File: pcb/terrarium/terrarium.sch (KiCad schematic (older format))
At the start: 22 parts, among them J3 Screw_Terminal_01x03, K3 SANYOU_SRD_Form_C, Q2 MMBT3904, U2 MOC3020M

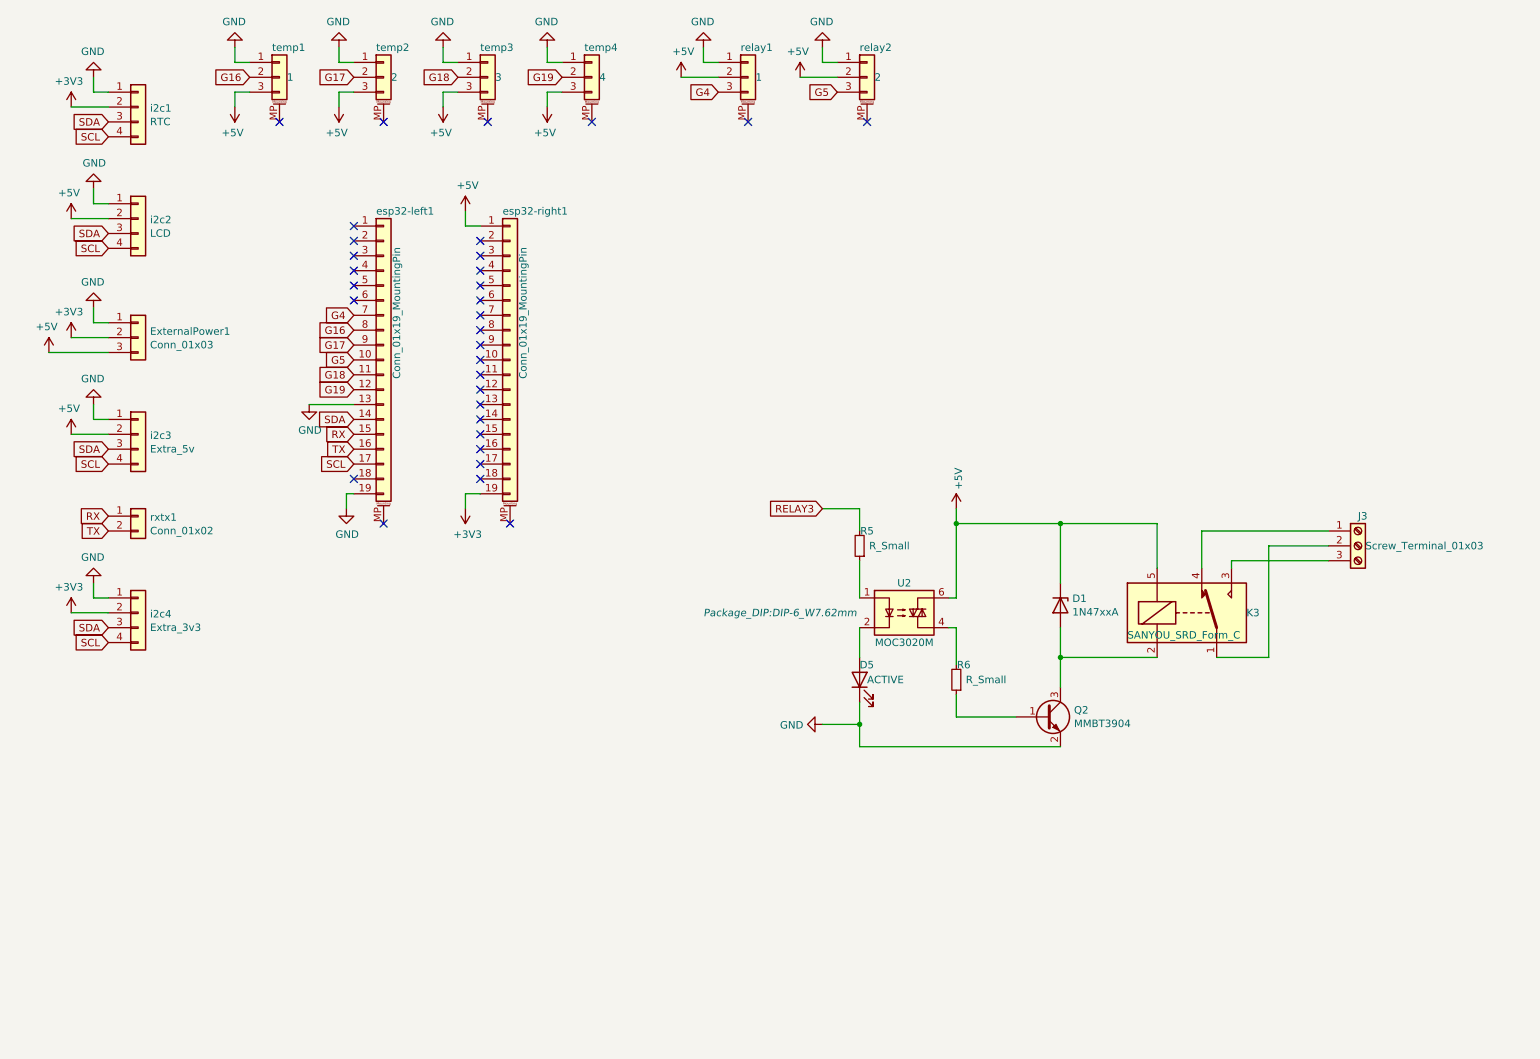
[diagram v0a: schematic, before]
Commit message: wip: update pcb
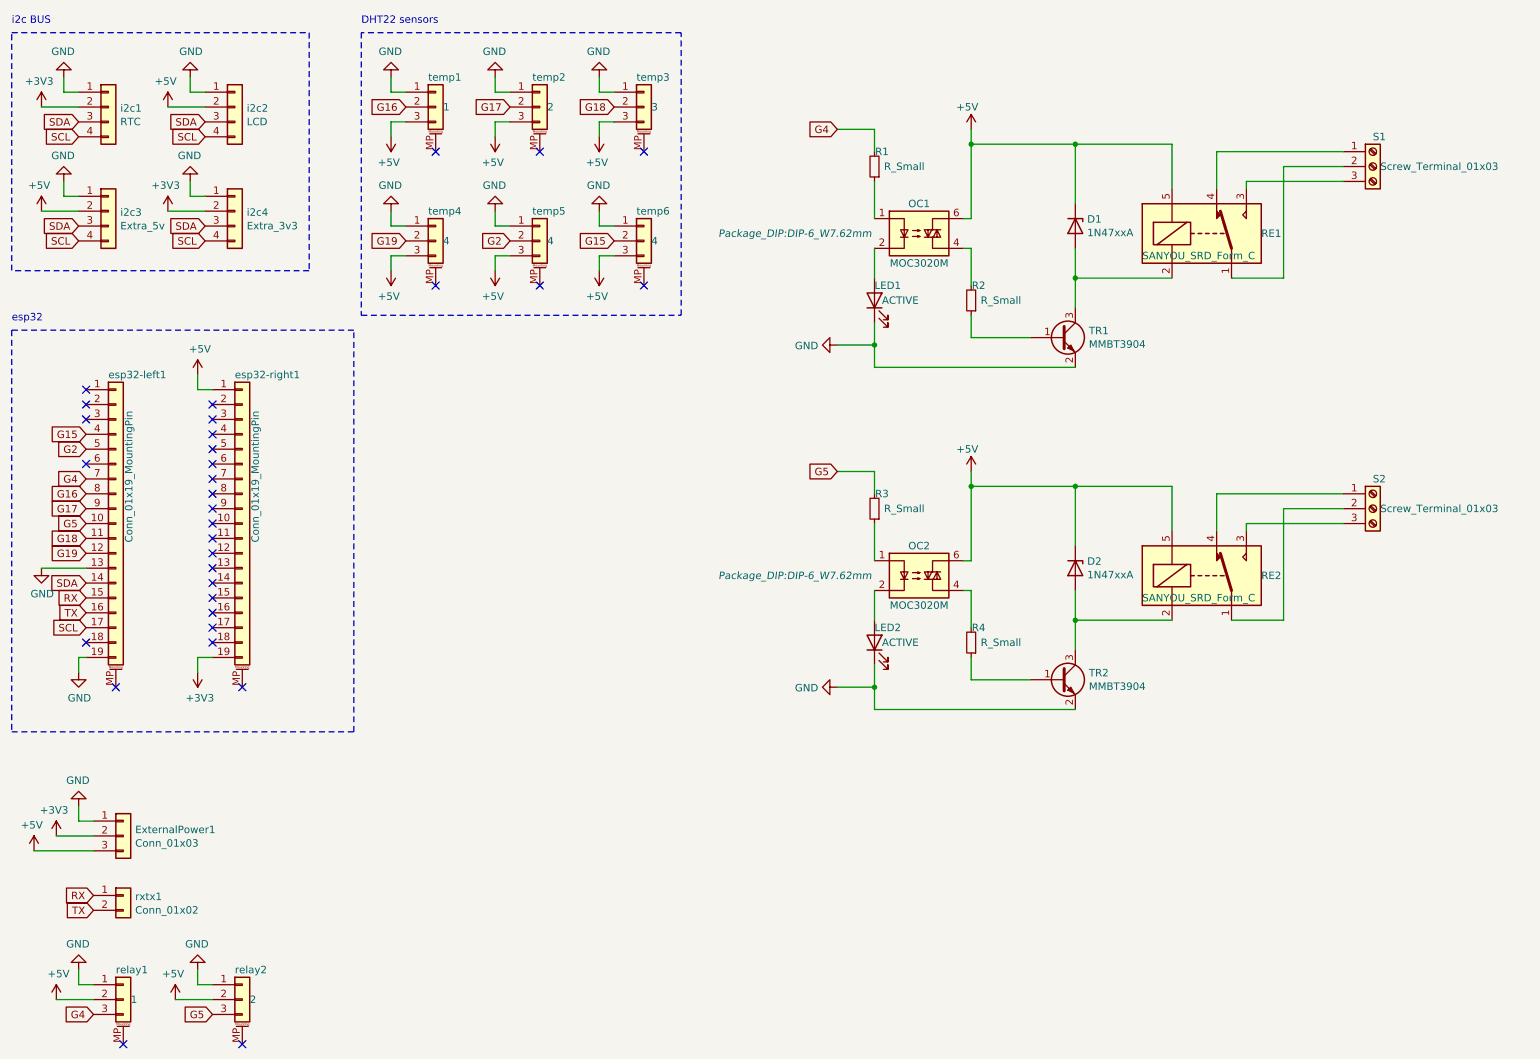
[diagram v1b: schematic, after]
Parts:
- added D2: 1N47xxA, Diode_THT:D_DO-41_SOD81_P7.62mm_Horizontal, symbol Diode:1N47xxA
- added LED2: ACTIVE, LED_THT:LED_D3.0mm_Clear, symbol Device:LED
- added OC2: MOC3020M, Package_DIP:DIP-6_W7.62mm, symbol Relay_SolidState:MOC3020M
- added R3, R4: R_Small, Resistor_THT:R_Axial_DIN0204_L3.6mm_D1.6mm_P2.54mm_Vertical, symbol Device:R_Small
- added RE2: SANYOU_SRD_Form_C, Relay_THT:Relay_SPDT_SANYOU_SRD_Series_Form_C, symbol Relay:SANYOU_SRD_Form_C
- added S2: Screw_Terminal_01x03, Connector_PinSocket_2.54mm:PinSocket_1x03_P2.54mm_Vertical, symbol Connector:Screw_Terminal_01x03
- added TR2: MMBT3904, Package_TO_SOT_THT:TO-92, symbol Transistor_BJT:MMBT3904
- added temp5, temp6: 4, Connector_JST:JST_XH_B3B-XH-AM_1x03_P2.50mm_Vertical, symbol Connector_Generic_MountingPin:Conn_01x03_MountingPin
- D1: footprint Diode_THT:D_DO-41_SOD81_P10.16mm_Horizontal -> Diode_THT:D_DO-41_SOD81_P7.62mm_Horizontal
- TR1: renamed from Q2; footprint Package_TO_SOT_SMD:SOT-23 -> Package_TO_SOT_THT:TO-92
- i2c2: footprint Connector_PinHeader_2.54mm:PinHeader_1x04_P2.54mm_Vertical -> Connector_JST:JST_XH_B4B-XH-AM_1x04_P2.50mm_Vertical
- temp1, temp2, temp3, temp4: footprint Connector_PinHeader_2.54mm:PinHeader_1x03_P2.54mm_Vertical -> Connector_JST:JST_XH_B3B-XH-AM_1x03_P2.50mm_Vertical
- renumbered D5 to LED1, U2 to OC1, R5 to R1, R6 to R2, K3 to RE1, J3 to S1
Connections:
- net RELAY3 is gone; now on net G4: R1.2
- net +5V: now also D2.1 (K), OC2.6, RE2.5, temp5.3 (Pin_3), temp6.3 (Pin_3)
- net G5: now also R3.2
- net GND: now also LED2.1 (K), TR2.2 (E), temp5.1 (Pin_1), temp6.1 (Pin_1)
- net G15: now reaches esp32-left1.4 (Pin_4)
- net G15: now also temp6.2 (Pin_2)
- net G2: now reaches esp32-left1.5 (Pin_5)
- net G2: now also temp5.2 (Pin_2)
- new net: RE2.1, S2.2 (Pin_2)
- new net: D2.2 (A), RE2.2, TR2.3 (C)
- new net: RE2.3, S2.3 (Pin_3)
- new net: RE2.4, S2.1 (Pin_1)
- new net: OC2.1, R3.1
- new net: LED2.2 (A), OC2.2
- new net: OC2.4, R4.2
- new net: R4.1, TR2.1 (B)
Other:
- note added: "DHT22 sensors"
- note added: "esp32"
- note added: "i2c BUS"
- moved on the sheet: D1, ExternalPower1, LED1, OC1, R1, R2, RE1, S1, TR1, esp32-left1, esp32-right1, i2c1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

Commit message: wip: pcb relay design
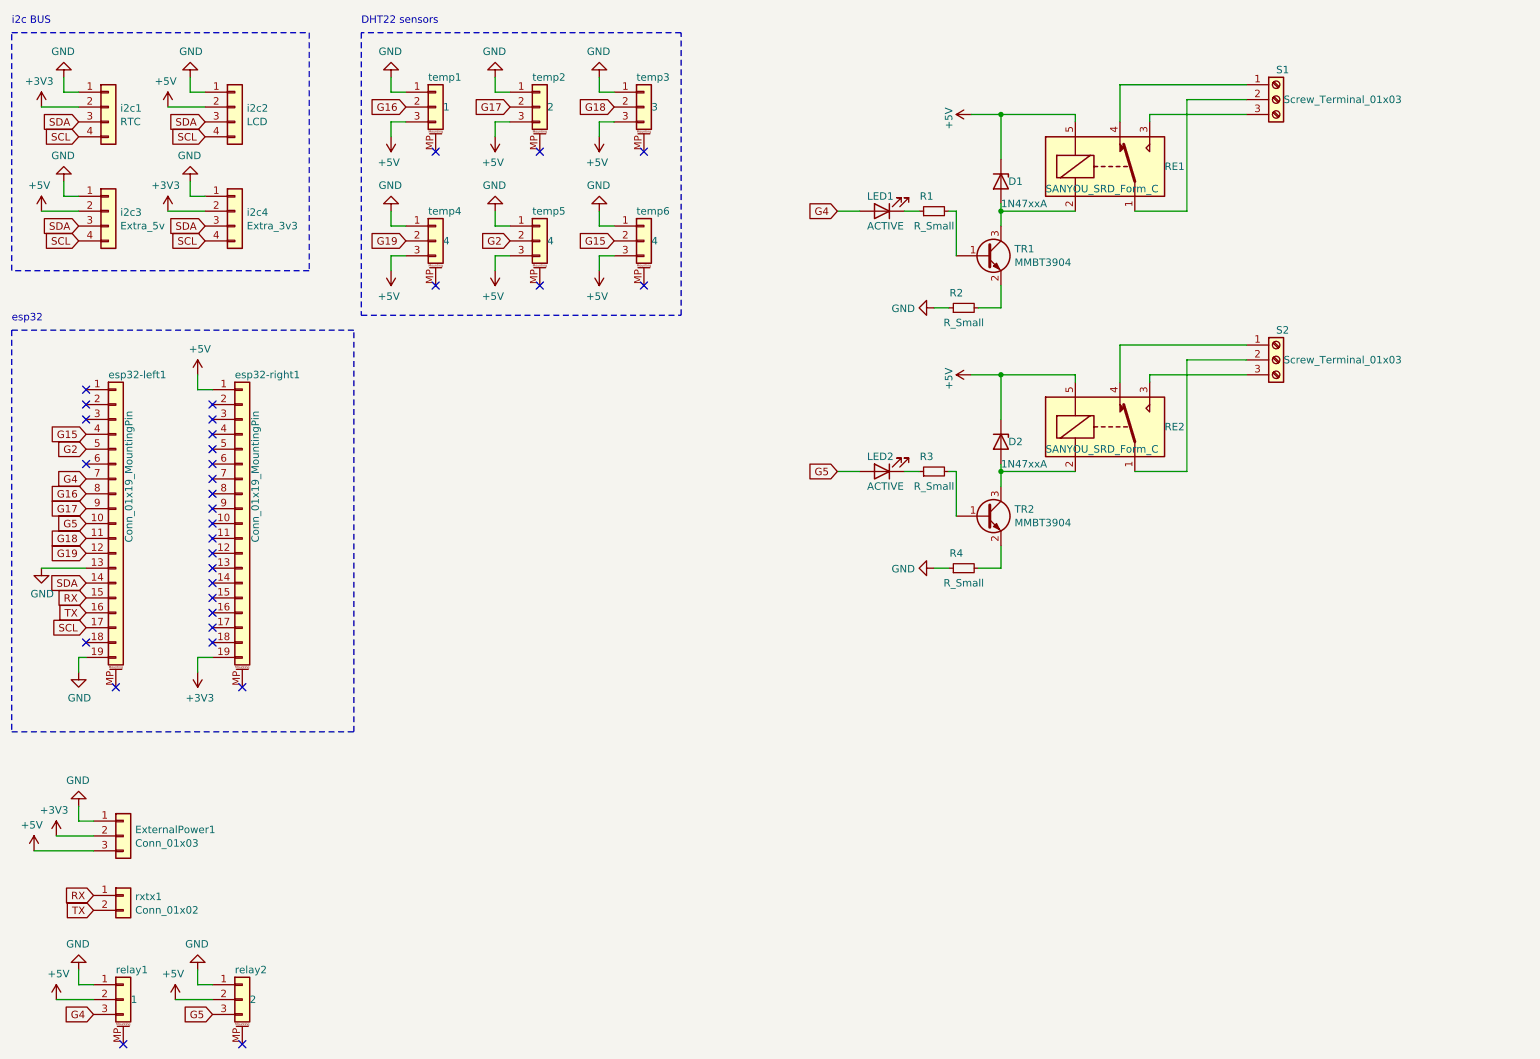
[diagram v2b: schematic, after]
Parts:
- removed OC1, OC2: MOC3020M, Package_DIP:DIP-6_W7.62mm, symbol Relay_SolidState:MOC3020M
- S1, S2: footprint Connector_PinSocket_2.54mm:PinSocket_1x03_P2.54mm_Vertical -> TerminalBlock:TerminalBlock_bornier-3_P5.08mm
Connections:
- net G4: now also LED1.2 (A); no longer R1.2
- net G5: now also LED2.2 (A); no longer R3.2
- net GND: now also R2.1, R4.1; no longer LED1.1 (K), LED2.1 (K), TR1.2 (E), TR2.2 (E)
- net at R1.1: now also LED1.1 (K)
- net at R2.2: now also TR1.2 (E)
- net at TR1.1 (B): now also R1.2; no longer R2.1
- net at R3.1: now also LED2.1 (K)
- net at R4.2: now also TR2.2 (E)
- net at TR2.1 (B): now also R3.2; no longer R4.1
